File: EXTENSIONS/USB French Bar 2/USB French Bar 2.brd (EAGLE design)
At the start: 50 x 50 mm, 11 parts, among them P1-GRD PTR1TP20SQ, P1-PLUS PTR1TP20SQ, P2-GRD PTR1TP20SQ, P2-PLUS PTR1TP20SQ, P3-GRD PTR1TP20SQ, P3-PLUS PTR1TP20SQ, X1 USB-A

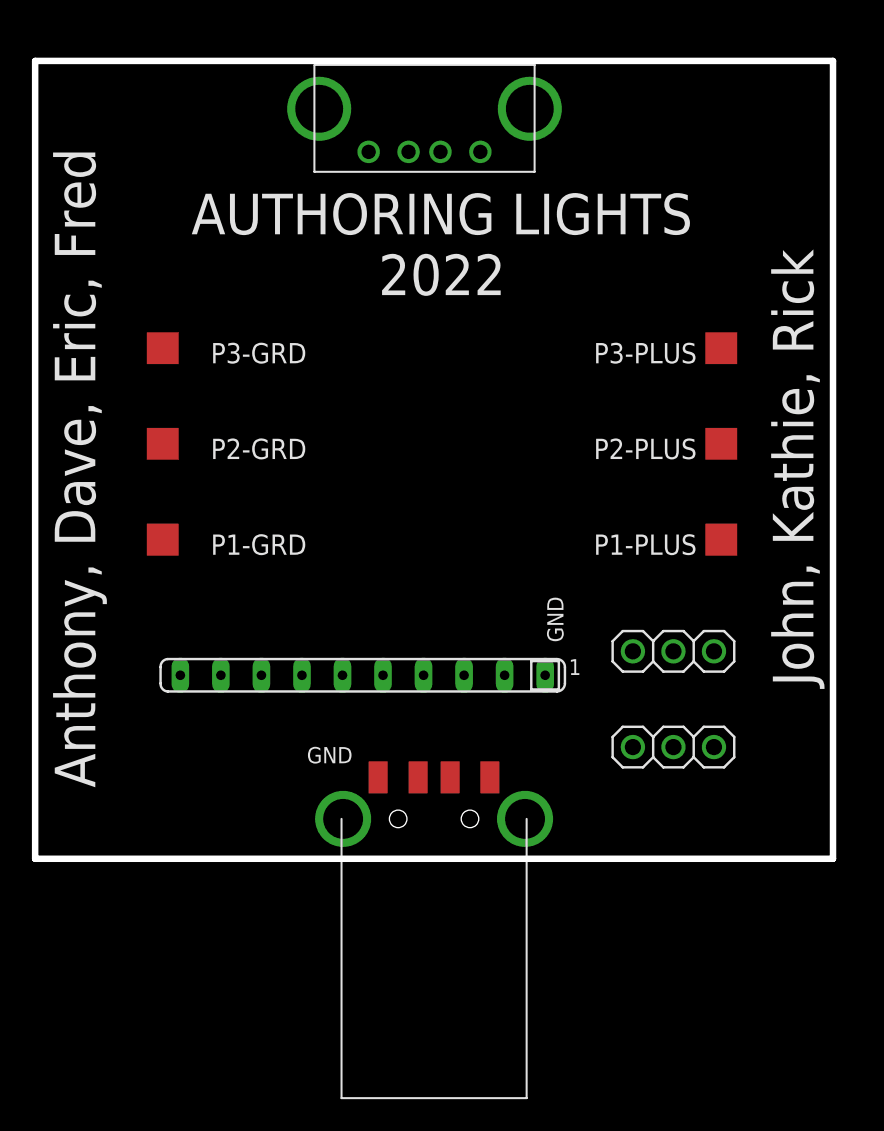
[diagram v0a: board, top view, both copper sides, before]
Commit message: more French usb 2
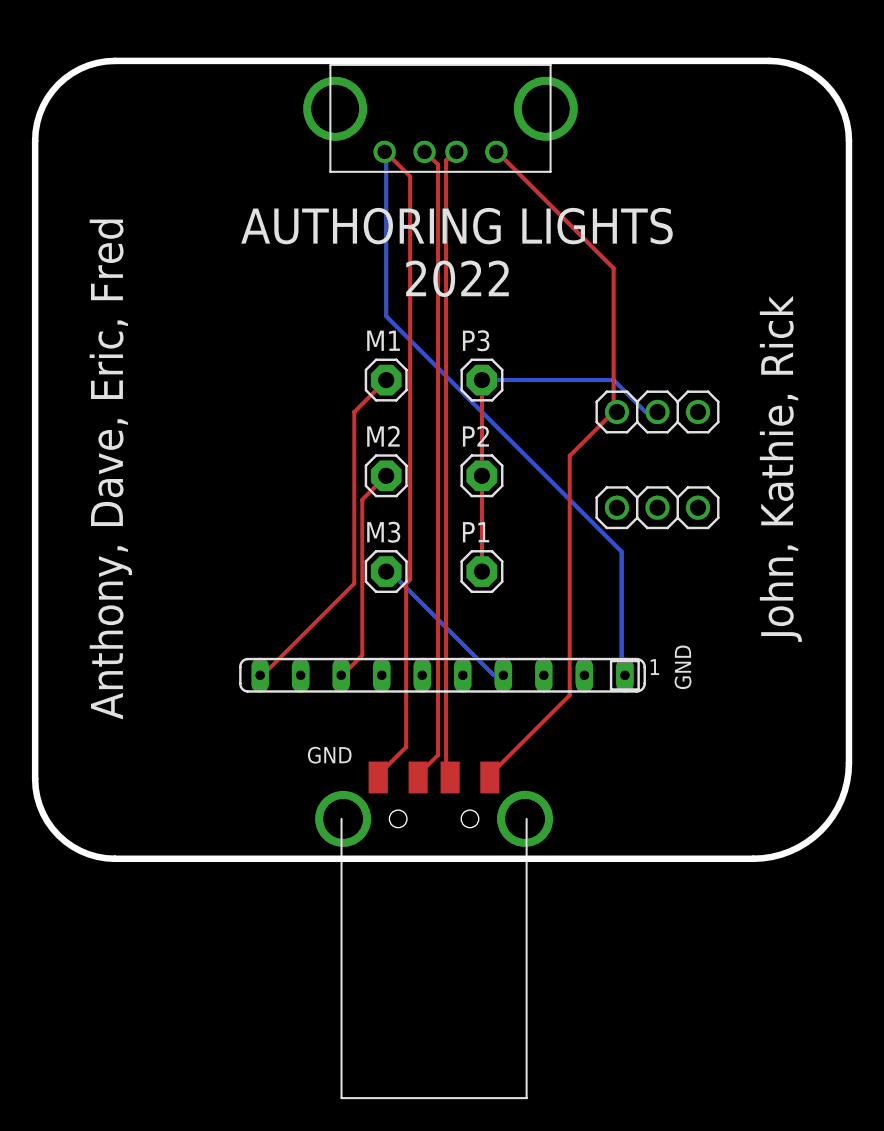
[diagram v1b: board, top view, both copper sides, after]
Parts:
- removed P1-GRD, P1-PLUS, P2-GRD, P2-PLUS, P3-GRD, P3-PLUS: PTR1TP20SQ, testpad:TP20SQ
- added M1, M2, M3, P1, P2, P3: (no value), adafruit:1X01
- moved JP1 15.0 mm to (39.0, 28.0)
- moved JP3 15.0 mm to (39.0, 22.0)
- moved RN1 5.00 mm to (25.5, 11.5)
- moved U$1 1.00 mm to (18.5, 43.0)
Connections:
- removed net N$7: JP1.2, P1-PLUS.TP, P2-PLUS.TP, P3-PLUS.TP
- new net N$8: JP1.2, P1.1, P2.1, P3.1
- net N$2: now also M1.1; no longer P1-GRD.TP
- net N$5: now also M2.1; no longer P2-GRD.TP
- net N$6: now also M3.1, RN1.4; no longer P3-GRD.TP, RN1.6
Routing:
- net N$1: track 0.00 -> 79.9 mm
- net VCC: track 0.00 -> 45.7 mm
- net N$3: track 0.00 -> 40.1 mm
- net N$4: track 0.00 -> 39.6 mm
- net N$8: track 0.00 -> 23.8 mm
- net N$2: track 0.00 -> 21.9 mm
- net N$5: track 0.00 -> 13.7 mm
- net N$6: track 0.00 -> 10.0 mm
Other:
- board size 50 x 50 mm -> 51 x 50 mm
